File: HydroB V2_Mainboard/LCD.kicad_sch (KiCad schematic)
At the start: 0 parts

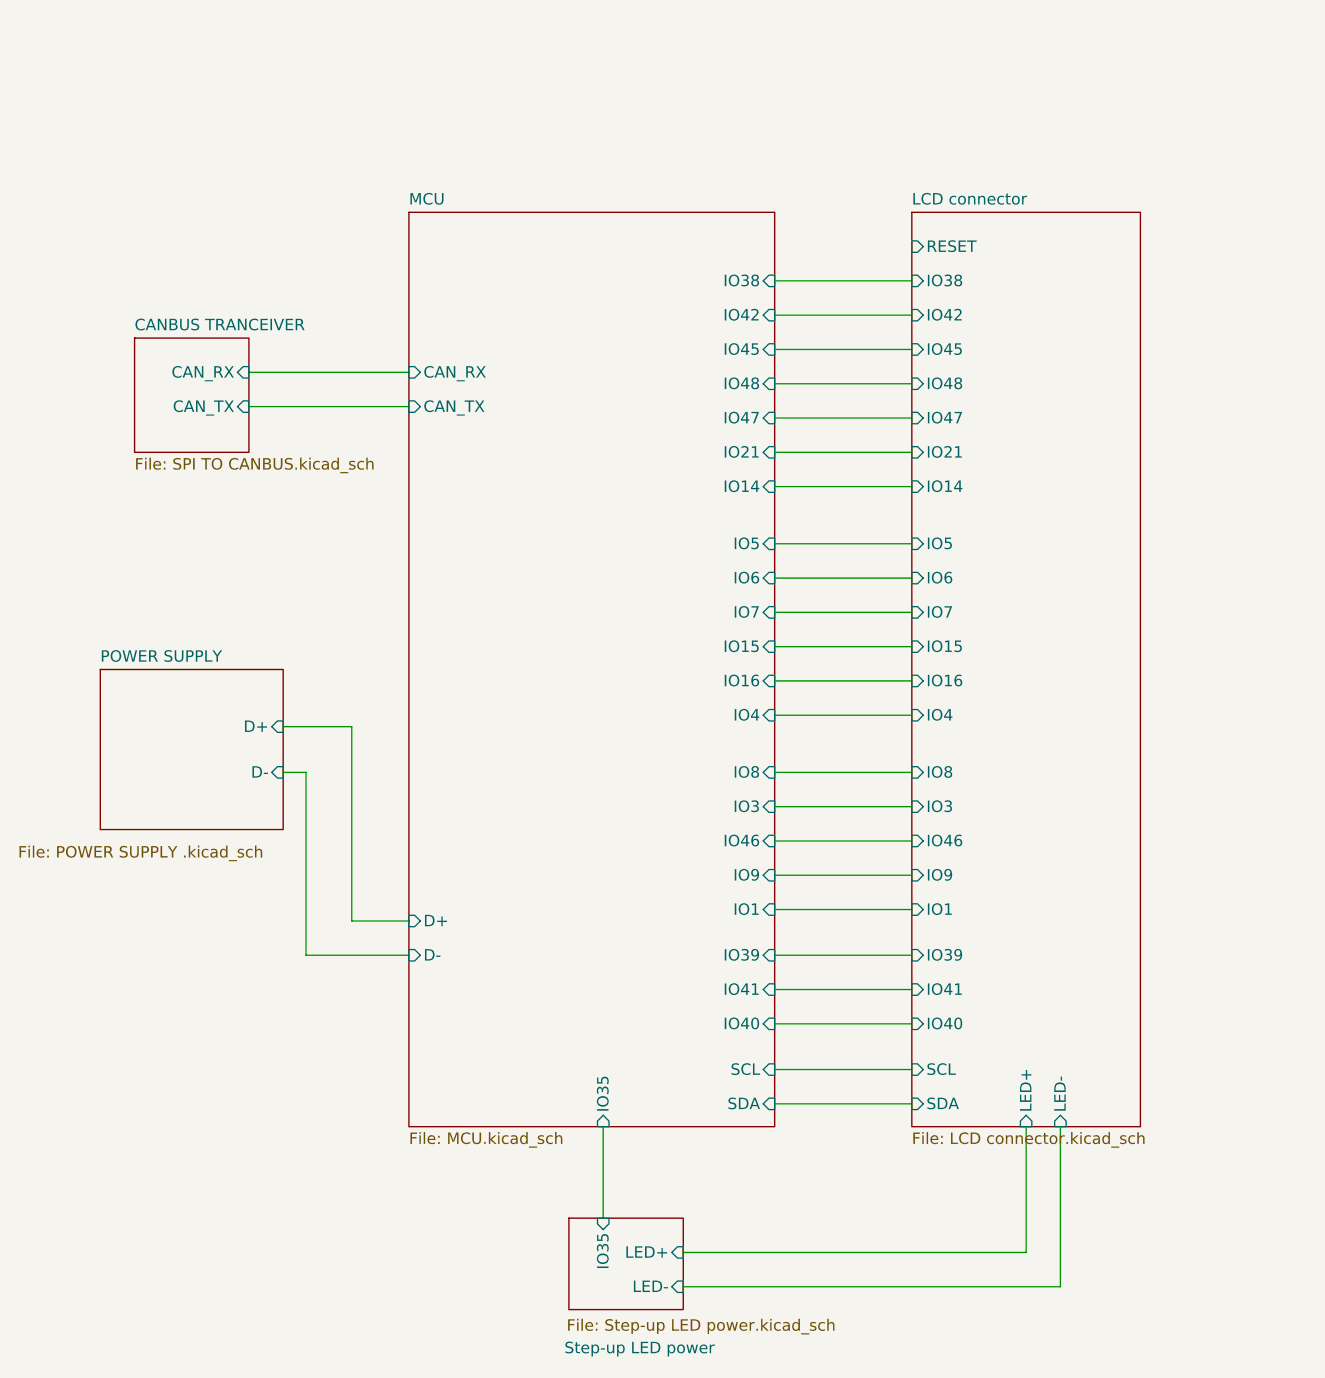
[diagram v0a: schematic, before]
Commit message: Schematic mainboard update
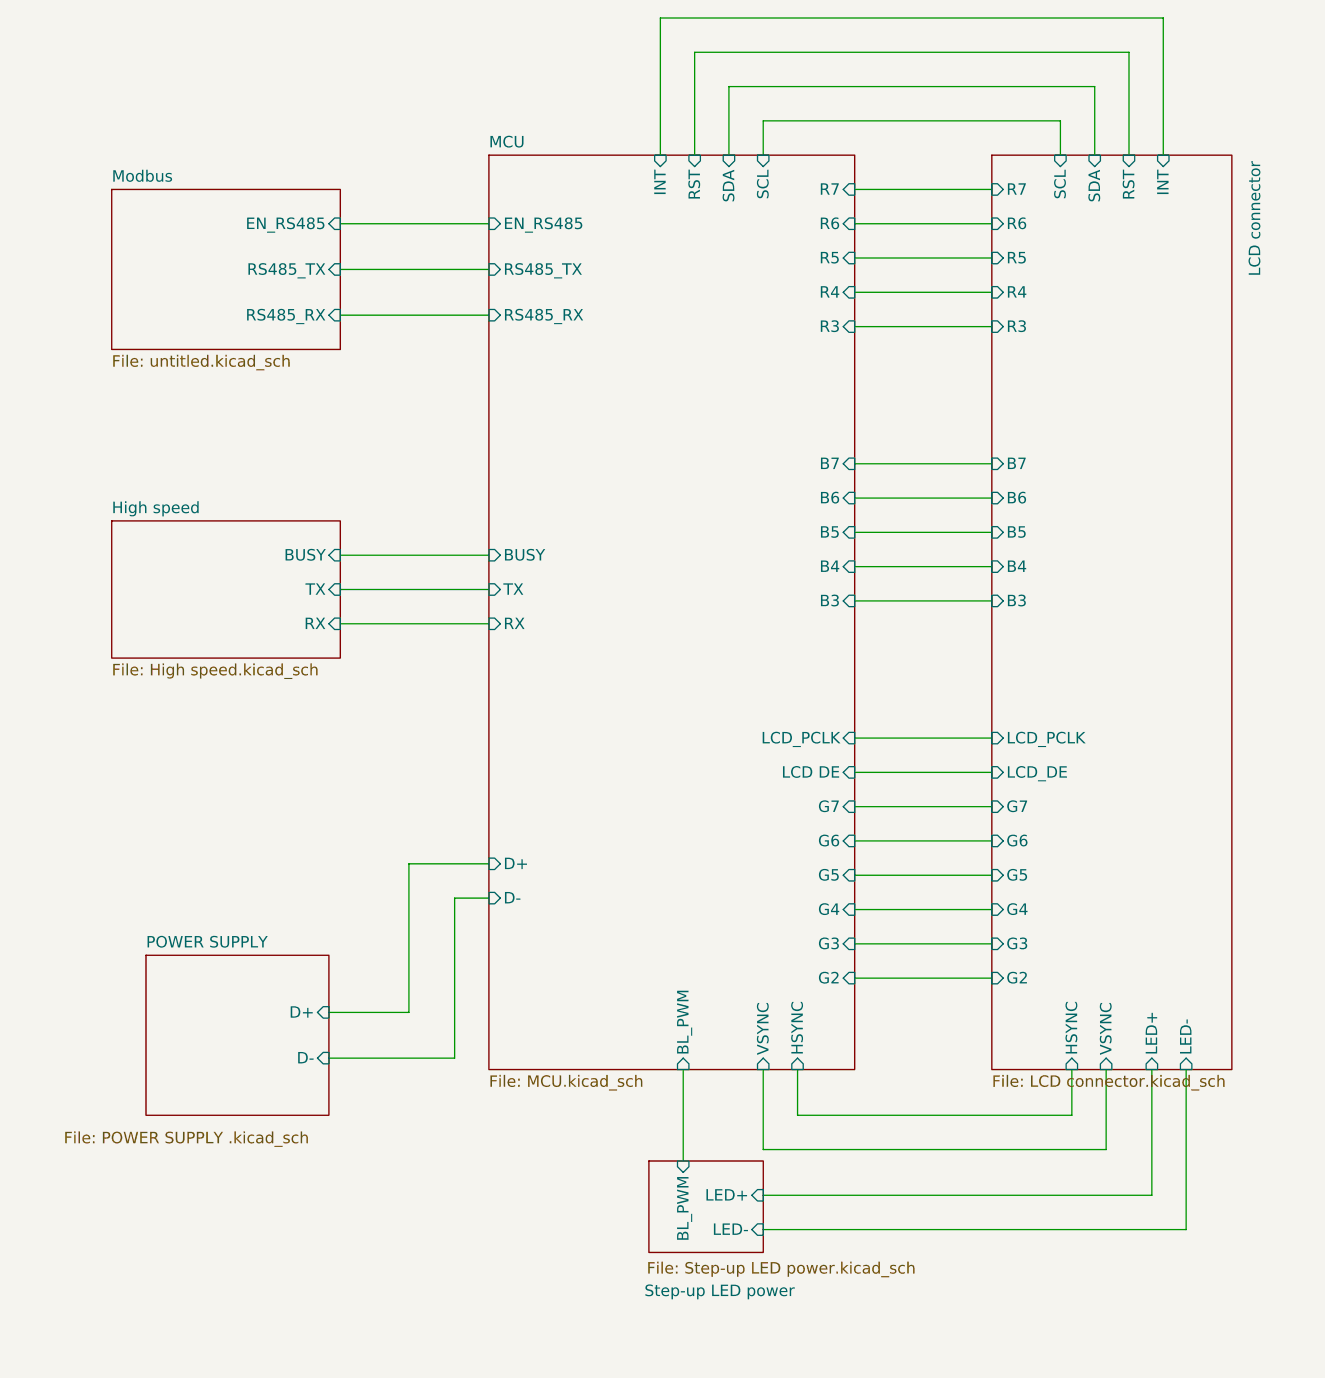
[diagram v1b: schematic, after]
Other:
- removed sheet CANBUS TRANCEIVER
- added sheet High speed  (High speed.kicad_sch)
- added sheet Modbus (untitled.kicad_sch)
- sheet LCD connector ports: added B3, B4, B5, B6, B7, G2, G3, G4, G5, G6, G7, HSYNC, INT, LCD_DE, LCD_PCLK, R3, R4, R5, R6, R7, RST, VSYNC; removed IO1, IO14, IO15, IO16, IO21, IO3, IO38, IO39, IO4, IO40, IO41, IO42, IO45, IO46, IO47, IO48, IO5, IO6, IO7, IO8, IO9, RESET
- sheet MCU ports: added B3, B4, B5, B6, B7, BL_PWM, BUSY, EN_RS485, G2, G3, G4, G5, G6, G7, HSYNC, INT, LCD DE, LCD_PCLK, R3, R4, R5, R6, R7, RS485_RX, RS485_TX, RST, RX, TX, VSYNC; removed CAN_RX, CAN_TX, IO1, IO14, IO15, IO16, IO21, IO3, IO35, IO38, IO39, IO4, IO40, IO41, IO42, IO45, IO46, IO47, IO48, IO5, IO6, IO7, IO8, IO9
- sheet Step-up LED power ports: added BL_PWM; removed IO35
